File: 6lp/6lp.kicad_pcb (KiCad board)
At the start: 2 copper layers, 25.4 x 27.9 mm, 34 parts, among them J1 MODULE_HEADER, T1 2450BM15A0015, U1 AT86RF233, X1 16.0000MF09Z-AC3

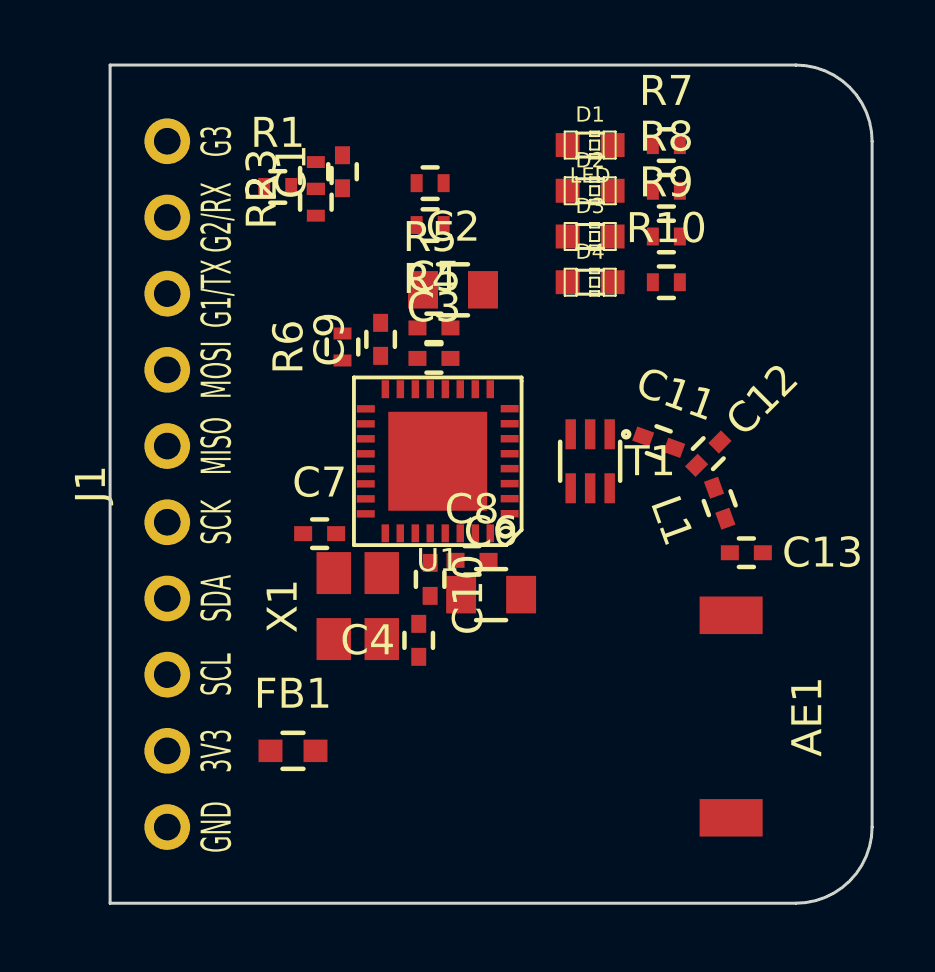
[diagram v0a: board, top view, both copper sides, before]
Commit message: closed project for review
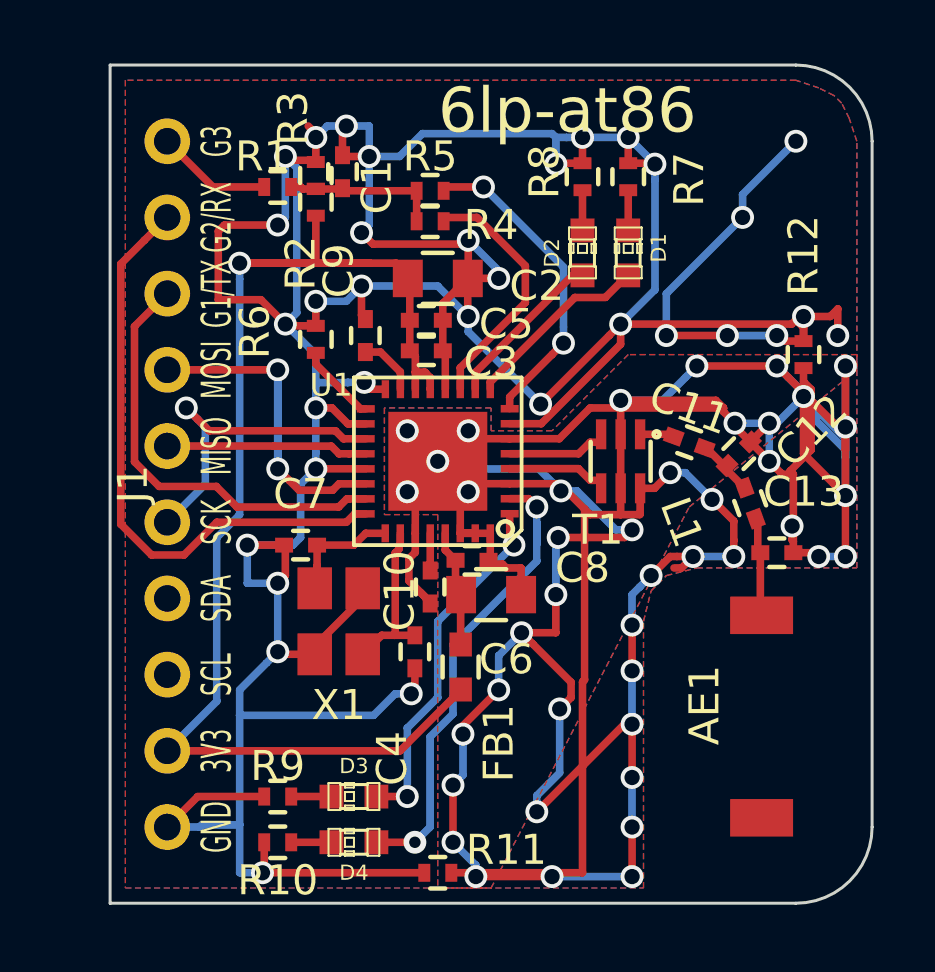
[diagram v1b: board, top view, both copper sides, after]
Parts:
- added R11: 0, Resistors_SMD:R_0402, F.Cu at (137.9, 126.0)
- added R12: 0, Resistors_SMD:R_0402, F.Cu at (150.1, 108.7)
- moved R10 22.7 mm to (132.6, 125.0), turned to 180 degrees
- moved R9 22.7 mm to (132.6, 123.4), turned to 180 degrees
- moved D3 20.3 mm to (135.1, 123.4), turned to 180 degrees
- moved D4 20.3 mm to (135.1, 125.0), turned to 180 degrees
- moved FB1 6.25 mm to (138.7, 119.1), turned to 90 degrees
- moved D1 3.81 mm to (144.3, 105.3), turned to 90 degrees
- moved R8 2.83 mm to (142.7, 102.8), turned to 90 degrees
- moved D2 2.09 mm to (142.7, 105.3), turned to 90 degrees
- moved R7 1.65 mm to (144.3, 102.8), turned to 90 degrees
- moved AE1 1.02 mm to (148.7, 120.8)
- moved C12 1.02 mm to (148.0, 112.0)
- moved L1 1.02 mm to (148.3, 113.7)
- moved C11 1.02 mm to (146.3, 111.6)
- moved C13 1.02 mm to (149.2, 115.3)
- moved T1 1.02 mm to (144.0, 112.3)
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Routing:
- net AGND: track 0.00 -> 173.4 mm, vias 0 -> 42
- net DGND: track 0.00 -> 158.6 mm, vias 0 -> 33
- net +3.3V: track 0.00 -> 44.6 mm, vias 0 -> 1
- net /INTERRUPT: track 0.00 -> 20.0 mm
- net /DIG4: track 0.00 -> 15.9 mm, vias 0 -> 2
- net /~CS: track 0.00 -> 14.5 mm
- net /MOSI: track 0.00 -> 13.3 mm, vias 0 -> 2
- net /DIG3: track 0.00 -> 12.0 mm, vias 0 -> 2
- net /SCLK: track 0.00 -> 11.0 mm, vias 0 -> 1
- net /~RESET: track 0.00 -> 10.6 mm, vias 0 -> 2
- net /SLP_TR: track 0.00 -> 8.52 mm
- net /MISO: track 0.00 -> 6.72 mm
- net /DIG1: track 0.00 -> 6.55 mm
- net /XTAL1: track 0.00 -> 5.54 mm
- net /DIG2: track 0.00 -> 5.47 mm
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- added copper zone on B.Cu, net AGND
- added copper zone on F.Cu, net AGND
- added copper zone on B.Cu, net DGND
- added copper zone on F.Cu, net DGND
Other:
- net class Default: clearance 0.254 -> 0.2032; via_dia 0.889 -> 0.762; via_drill 0.635 -> 0.508
- rule trace_clearance: 0.254 -> 0.2032
- rule via_min_size: 0.889 -> 0.762
- board text added: "6lp-at86"
